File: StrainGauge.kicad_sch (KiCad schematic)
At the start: 34 parts, among them J1 Conn_01x04, J2 502585-0470, U1 INA333xxDGK, U2 REF2025, U3 OPA310xDBV, U4 OPA310xDBV

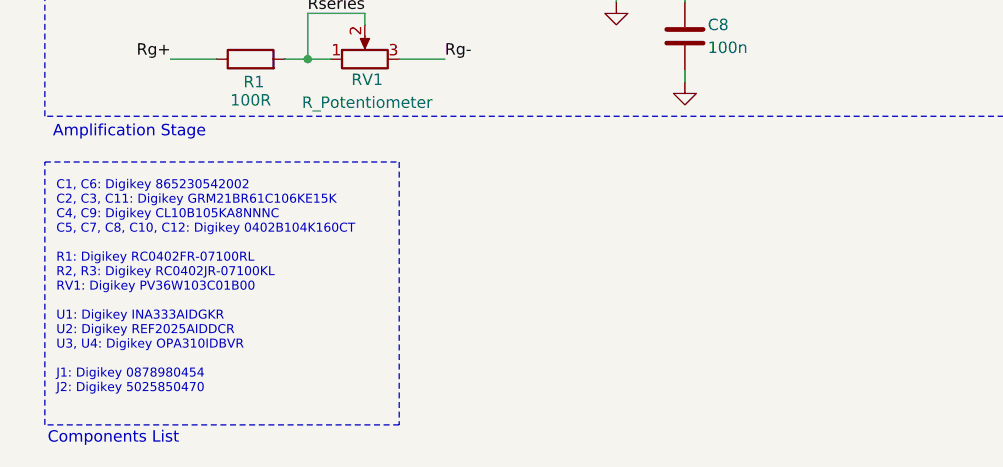
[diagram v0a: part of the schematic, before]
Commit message: small fixes
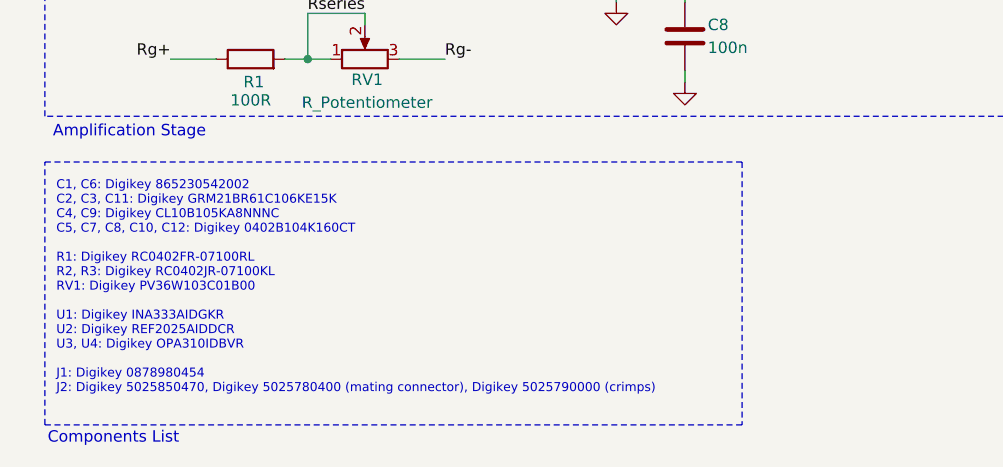
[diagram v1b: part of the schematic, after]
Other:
- note added: "C1, C6: Digikey 865230542002 C2, C3, C11: Digikey GRM21BR61C106KE15K C4, C9: Digikey CL10B105KA8NNNC C5, C7, C8, C10, C12: Digikey 0402B104K160CT R1: Digikey RC0402FR-07100RL R2, R3: Digikey RC0402JR-07100KL RV1: Digikey PV36W103C01B00 U1: Digikey INA333AIDGKR U2: Digikey REF2025AIDDCR U3, U4: Digikey OPA310IDBVR J1: Digikey 0878980454 J2: Digikey 5025850470, Digikey 5025780400 (mating connector)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"
- note removed: "C1, C6: Digikey 865230542002 C2, C3, C11: Digikey GRM21BR61C106KE15K C4, C9: Digikey CL10B105KA8NNNC C5, C7, C8, C10, C12: Digikey 0402B104K160CT R1: Digikey RC0402FR-07100RL R2, R3: Digikey RC0402JR-07100KL RV1: Digikey PV36W103C01B00 U1: Digikey INA333AIDGKR U2: Digikey REF2025AIDDCR U3, U4: Digikey OPA310IDBVR J1: Digikey 0878980454 J2: Digikey 5025850470"
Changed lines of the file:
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@@
 	(rectangle
 		(start 16.51 158.75)
-		(end 55.88 187.96)
+		(end 93.98 187.96)
 		(stroke
 			(width 0)
@@
 		)
 	)
-	(text "C1, C6: Digikey 865230542002\nC2, C3, C11: Digikey GRM21BR61C106KE15K\nC4, C9: Digikey CL10B105KA8NNNC\nC5, C7, C8, C10, C12: Digikey 0402B104K160CT\n\nR1: Digikey RC0402FR-07100RL\nR2, R3: Digikey RC0402JR-07100KL\nRV1: Digikey PV36W103C01B00\n\nU1: Digikey INA333AIDGKR\nU2: Digikey REF2025AIDDCR\nU3, U4: Digikey OPA310IDBVR\n\nJ1: Digikey 0878980454\nJ2: Digikey 5025850470"
+	(text "C1, C6: Digikey 865230542002\nC2, C3, C11: Digikey GRM21BR61C106KE15K\nC4, C9: Digikey CL10B105KA8NNNC\nC5, C7, C8, C10, C12: Digikey 0402B104K160CT\n\nR1: Digikey RC0402FR-07100RL\nR2, R3: Digikey RC0402JR-07100KL\nRV1: Digikey PV36W103C01B00\n\nU1: Digikey INA333AIDGKR\nU2: Digikey REF2025AIDDCR\nU3, U4: Digikey OPA310IDBVR\n\nJ1: Digikey 0878980454\nJ2: Digikey 5025850470, Digikey 5025780400 (mating connector), Digikey 5025790000 (crimps)"
 		(exclude_from_sim no)
 		(at 17.78 172.72 0)
